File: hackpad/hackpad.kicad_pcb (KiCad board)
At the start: 2 copper layers, 57 x 81 mm, 10 parts, among them SW1 SW_Push, SW10 SW_Push, SW2 SW_Push, SW3 SW_Push, SW4 SW_Push, SW5 SW_Push, SW6 SW_Push, SW7 SW_Push, SW9 SW_Push, U1 MOUDLE-SEEEDUINO-XIAO

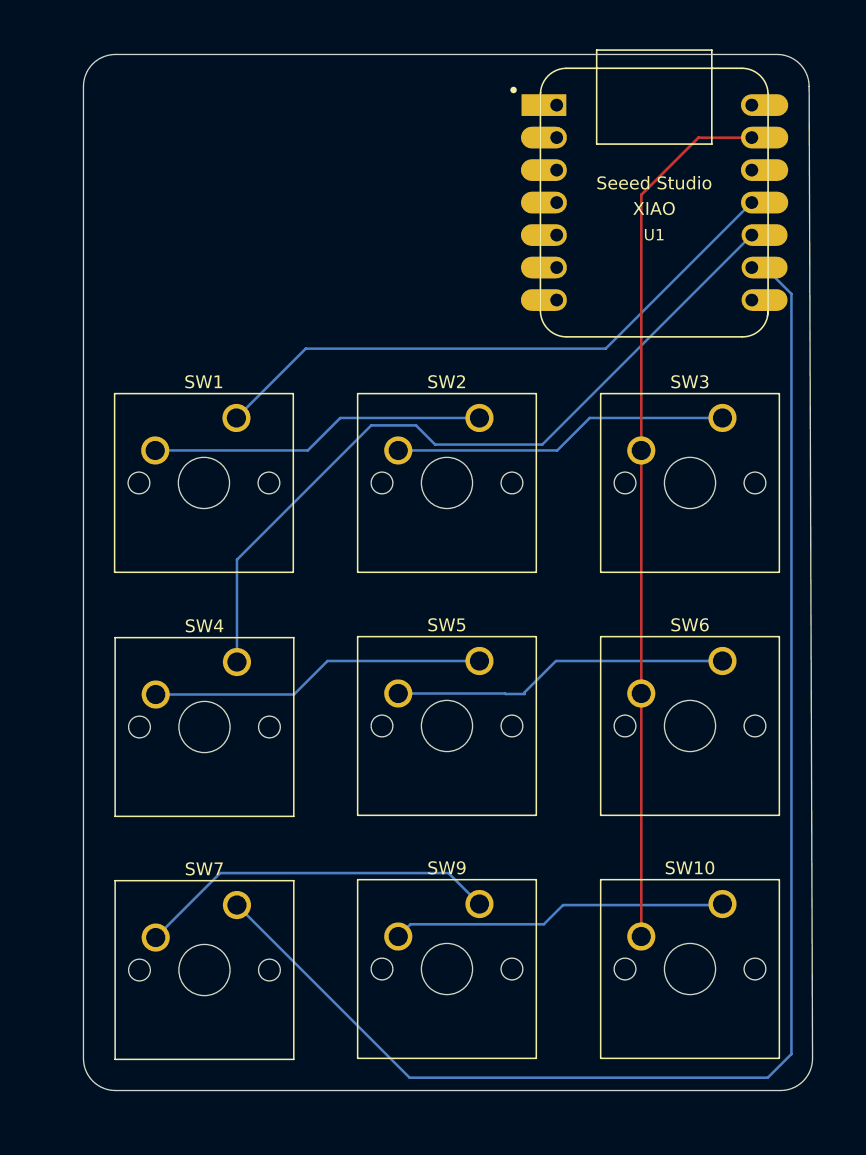
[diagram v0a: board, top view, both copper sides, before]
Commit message: Update
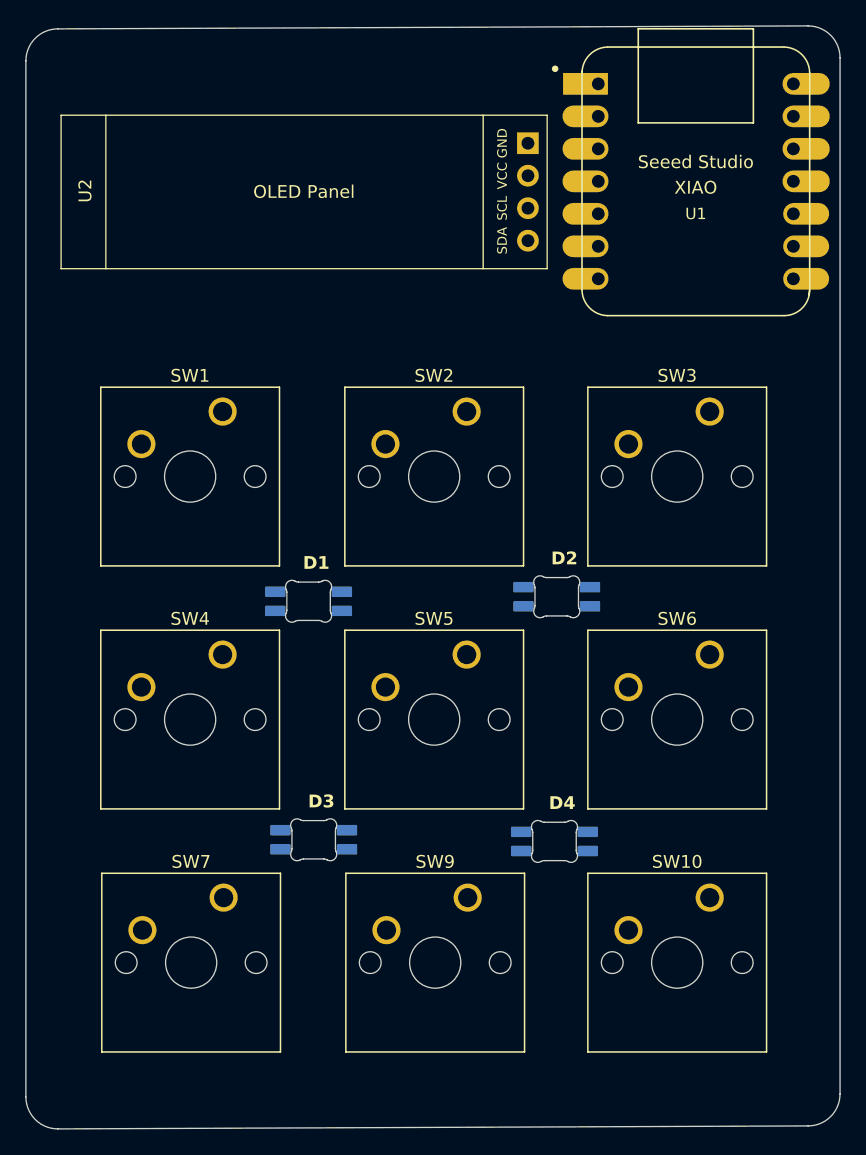
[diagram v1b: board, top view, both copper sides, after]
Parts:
- added D1: SK6812MINI-E, footprints:SK6812MINI-E_fixed, F.Cu at (174.1, 84.9)
- added D2: SK6812MINI-E, footprints:SK6812MINI-E_fixed, F.Cu at (193.5, 84.5)
- added D3: SK6812MINI-E, footprints:SK6812MINI-E_fixed, F.Cu at (174.5, 103.5)
- added D4: SK6812MINI-E, footprints:SK6812MINI-E_fixed, F.Cu at (193.3, 103.6)
- added U2: ~, OLED:SSD1306-0.91-OLED-4pin-128x32, F.Cu at (154.8, 46.8)
- moved U1 3.65 mm to (204.4, 51.9)
- moved SW4 1.26 mm to (167.4, 88.9)
- moved SW7 1.19 mm to (167.5, 107.9)
- moved SW1 1.19 mm to (167.4, 69.9)
- moved SW10 1.12 mm to (205.5, 107.9)
- moved SW2 1.12 mm to (186.5, 69.9)
- moved SW3 1.12 mm to (205.5, 69.9)
- moved SW5 1.12 mm to (186.5, 88.9)
- moved SW6 1.12 mm to (205.5, 88.9)
- moved SW9 1.05 mm to (186.5, 107.9)
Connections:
- U1 pad 12: unconnected-(U1-3V3-Pad12) -> /OLED VCC
- U1 pad 14: unconnected-(U1-5V-Pad14) -> /LED VDD
- U1 pad 2: unconnected-(U1-PA4_A1_D1-Pad2) -> Net-(D1-DIN)
- U1 pad 5: unconnected-(U1-PA8_A4_D4_SDA-Pad5) -> /<NO NET>
- U1 pad 6: unconnected-(U1-PA9_A5_D5_SCL-Pad6) -> /OLED SCL
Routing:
- net Net-(U1-PA7_A8_D8_SCK): track 114.0 -> 0.00 mm
- net GND: track 68.5 -> 0.00 mm
- net Net-(U1-PA5_A9_D9_MISO): track 60.0 -> 0.00 mm
- net Net-(U1-PA6_A10_D10_MOSI): track 47.3 -> 0.00 mm
- net Net-(SW7-Pad2): track 28.4 -> 0.00 mm
- net Net-(SW4-Pad2): track 27.1 -> 0.00 mm
- net Net-(SW5-Pad2): track 26.9 -> 0.00 mm
- net Net-(SW2-Pad2): track 26.4 -> 0.00 mm
- net Net-(SW1-Pad2): track 26.4 -> 0.00 mm
- net Net-(SW10-Pad1): track 26.4 -> 0.00 mm
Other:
- board size 57 x 81 mm -> 63.7 x 86.2 mm
